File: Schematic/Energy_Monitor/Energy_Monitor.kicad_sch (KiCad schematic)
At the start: 10 parts, among them J1 I2C LCD, J2 SD Card Module, J3 RTC, J4 PZEM-004T, SW1 SW_SPDT, U1 L7805, U2 LM2596, U3 Level_Shifter, U4 ESP32-WROOM-32

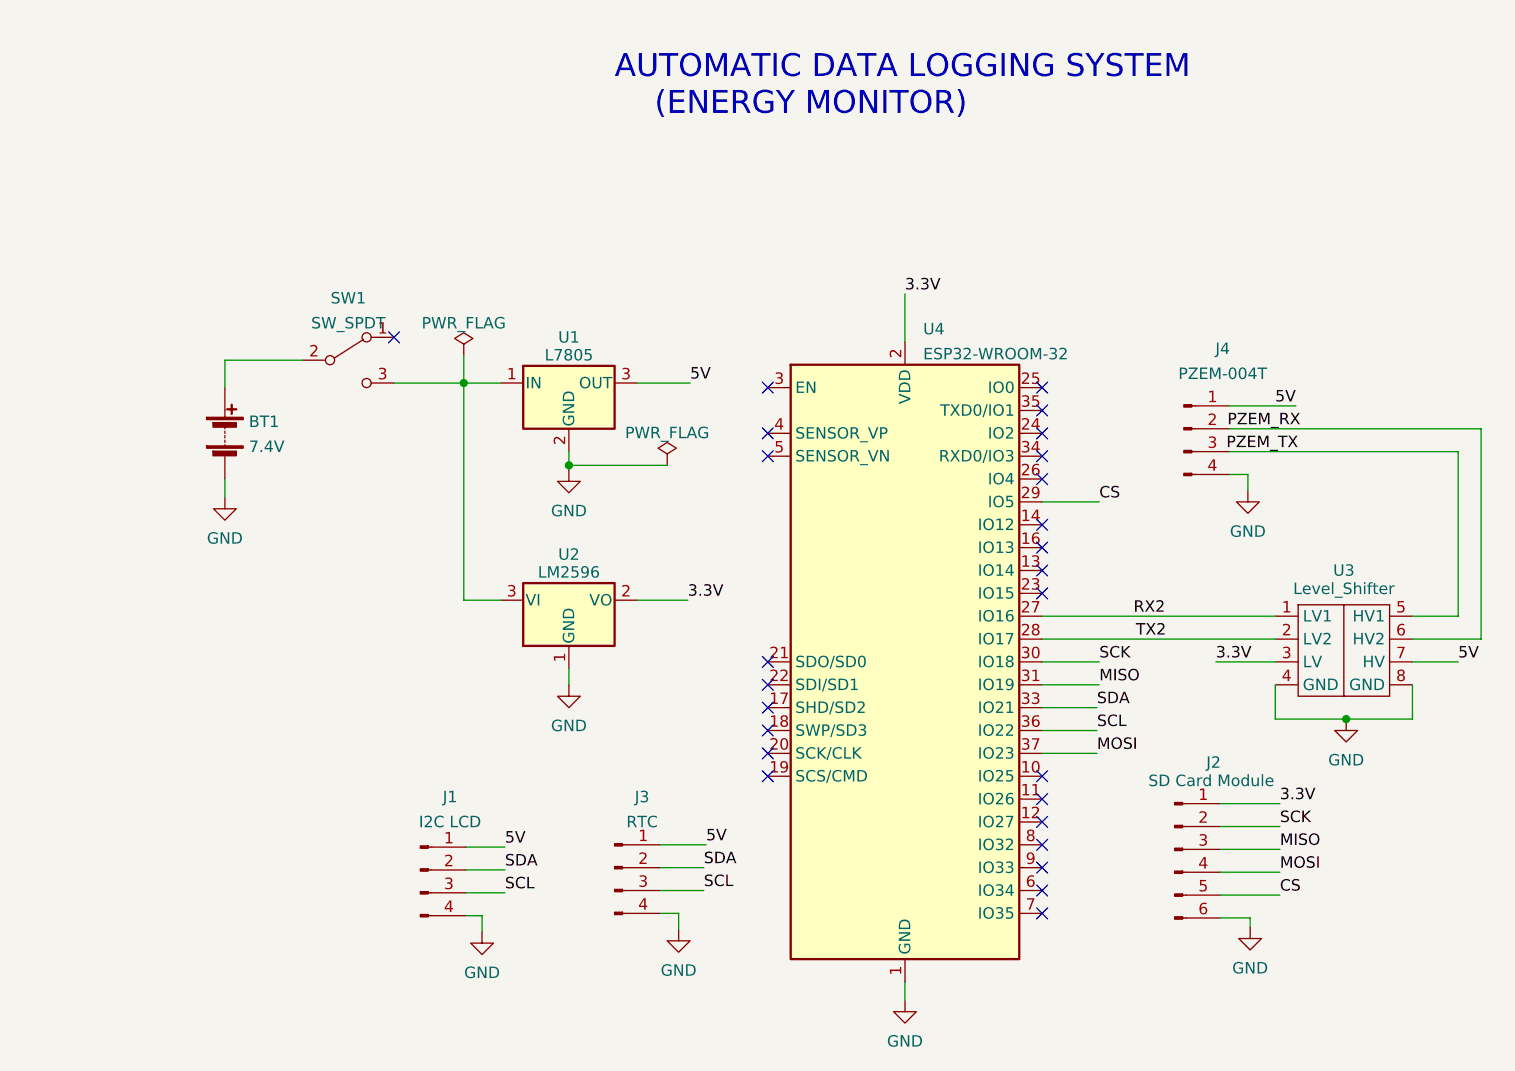
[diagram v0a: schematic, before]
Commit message: Add files via upload
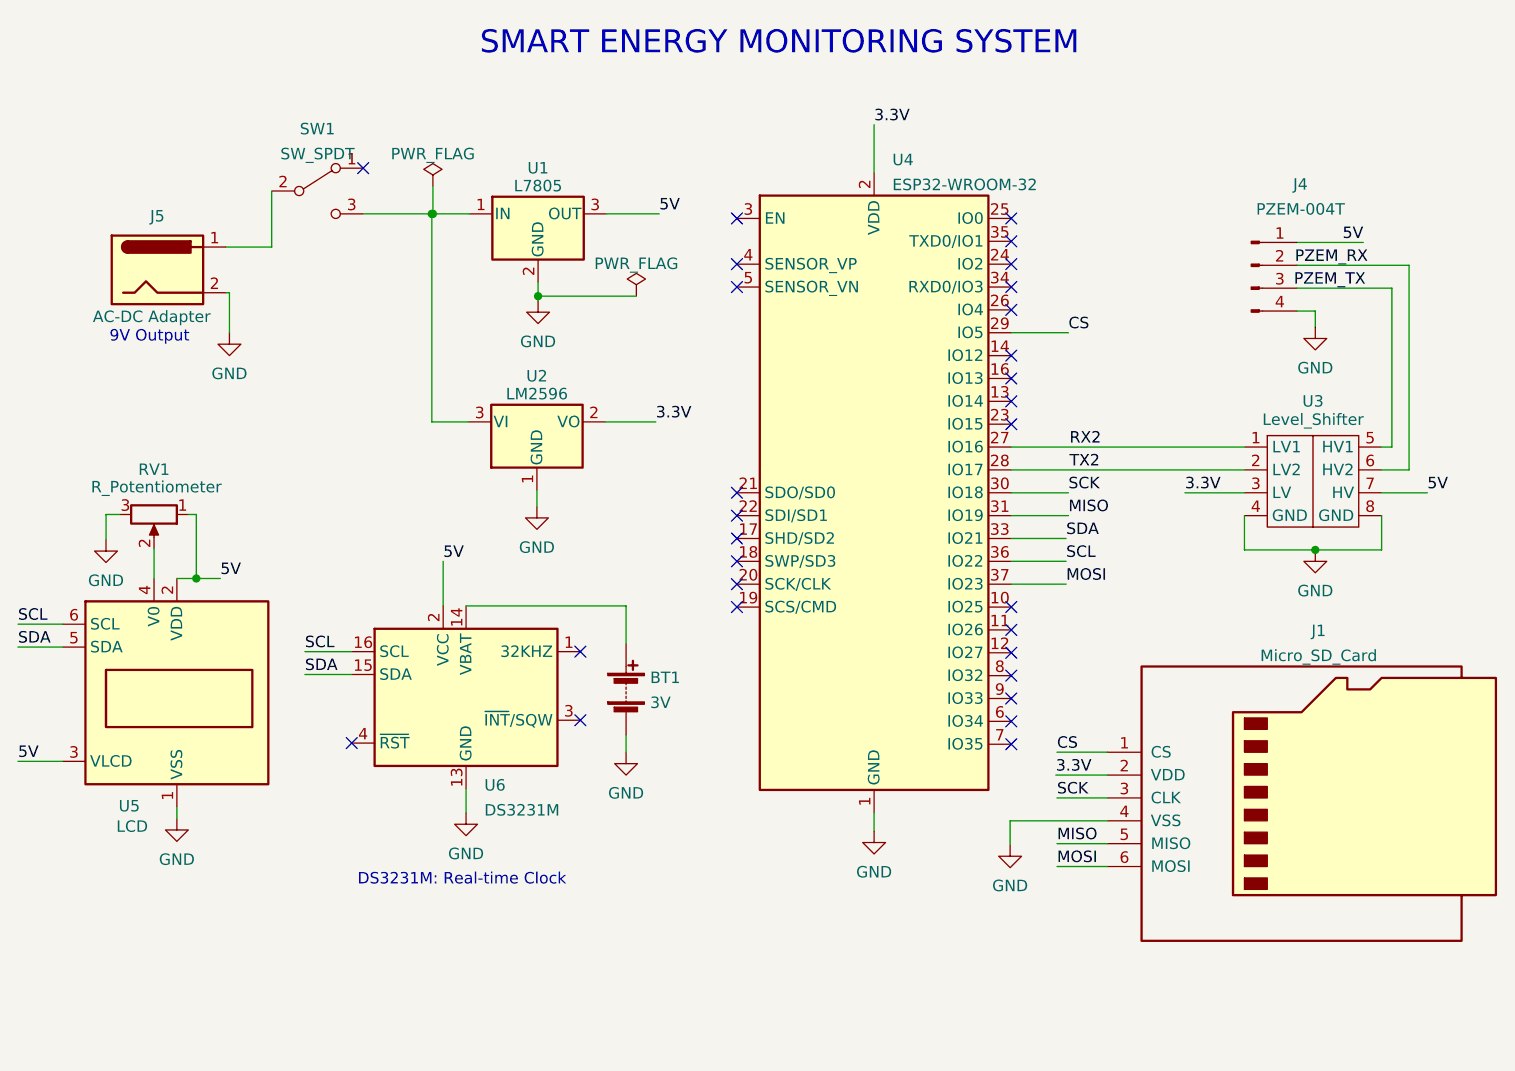
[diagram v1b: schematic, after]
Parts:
- removed J1: I2C LCD, symbol Connector:Conn_01x04_Male
- removed J2: SD Card Module, symbol Connector:Conn_01x06_Male
- removed J3: RTC, symbol Connector:Conn_01x04_Male
- added J1: Micro_SD_Card, symbol Connector:Micro_SD_Card
- added J5: AC-DC Adapter, symbol Connector:Jack-DC
- added RV1: R_Potentiometer, symbol Device:R_Potentiometer
- added U5: LCD, Display:EA_T123X-I2C, symbol Display_Character:EA_T123X-I2C
- added U6: DS3231M, Package_SO:SOIC-16W_7.5x10.3mm_P1.27mm, symbol Timer_RTC:DS3231M
- BT1: value 7.4V -> 3V
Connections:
- net 3.3V: now also J1.2 (VDD)
- net 5V: now also RV1.1, U5.2 (VDD), U5.3 (VLCD), U6.2 (VCC)
- net CS: now also J1.1 (CS)
- net GND: now also J1.4 (VSS), J5.2, RV1.3, U5.1 (VSS), U6.10 (GND), U6.11 (GND), U6.12 (GND), U6.13 (GND), U6.5 (GND), U6.6 (GND), U6.7 (GND), U6.8 (GND), U6.9 (GND)
- net MISO: now also J1.5 (MISO)
- net MOSI: now also J1.6 (MOSI)
- net SCK: now also J1.3 (CLK)
- net SCL: now also U5.6 (SCL), U6.16 (SCL)
- net SDA: now also U5.5 (SDA), U6.15 (SDA)
- net at BT1.1 (+): now also U6.14 (VBAT); no longer SW1.2 (B)
- new net: RV1.2, U5.4 (V0)
- new net: J5.1, SW1.2 (B)
- no-connect marks 26 -> 29
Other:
- note added: "9V Output"
- note added: "DS3231M: Real-time Clock"
- note added: "SMART ENERGY MONITORING SYSTEM"
- note removed: "AUTOMATIC DATA LOGGING SYSTEM (ENERGY MONITOR)"
- moved on the sheet: J4, SW1, U1, U2, U3, U4
